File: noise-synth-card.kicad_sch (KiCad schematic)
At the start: 23 parts, among them J11 Blend Out, J4 power, M1 imogen-wren-card, U1 HEF4093B, U2 TL074, U3 TL074, U4 TL074

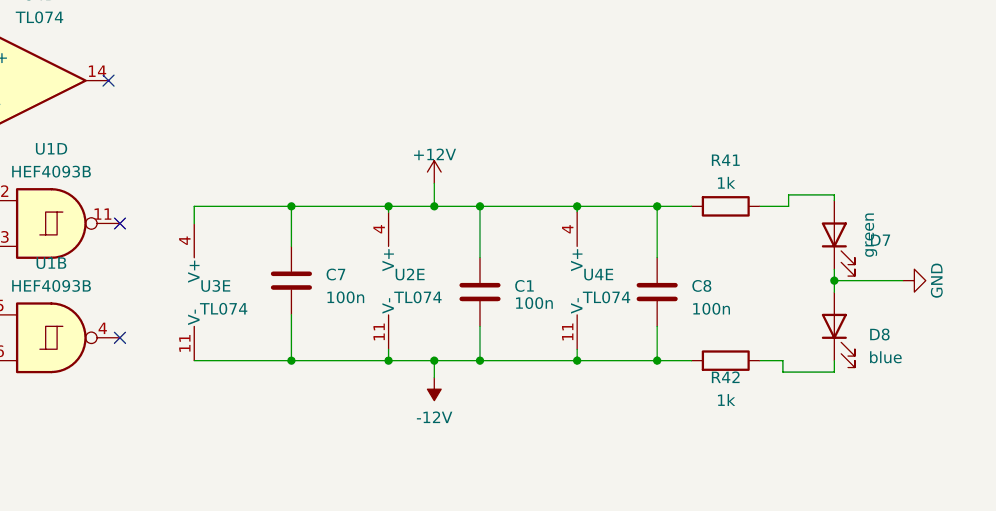
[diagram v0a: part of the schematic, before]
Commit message: dfgdrfghdf
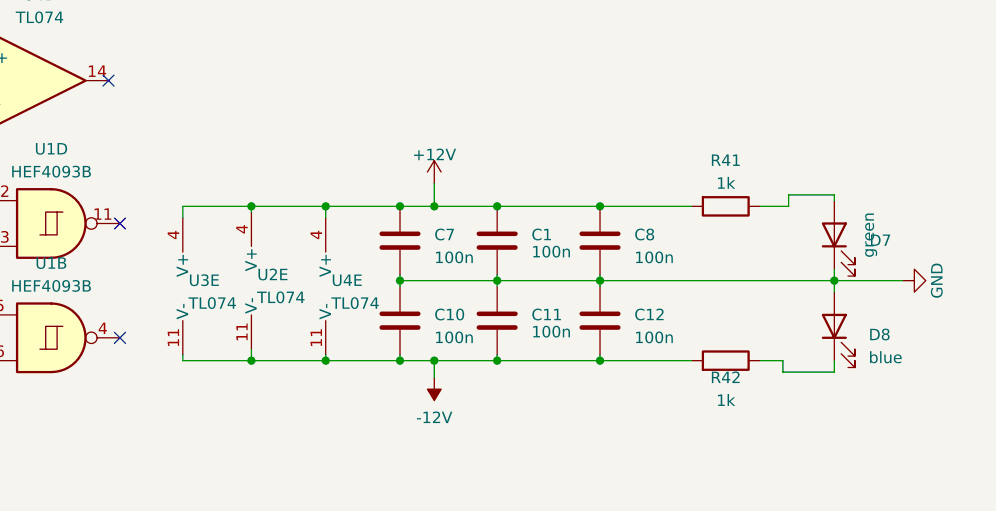
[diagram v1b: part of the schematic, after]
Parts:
- added C10, C11, C12: 100n, 000_Capacitors_Immo:C_0805_2012_HandSolder_kawaii, symbol 000_Capacitor_Film_Immo:100n
- M1: footprint 000_Modules_Immo:imogen-wren-card -> 000_Modules_Immo:credit-card-screws
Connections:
- net -12V: now also C10.2, C11.2, C12.2; no longer C1.2, C7.2, C8.2
- net GND: now also C1.2, C7.2, C8.2, C10.1, C11.1, C12.1
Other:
- moved on the sheet: C1, C7, C8, U2E, U3E, U4E
